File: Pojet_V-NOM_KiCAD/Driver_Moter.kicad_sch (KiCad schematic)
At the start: 3 parts, among them U701 ZXBM5210-SP

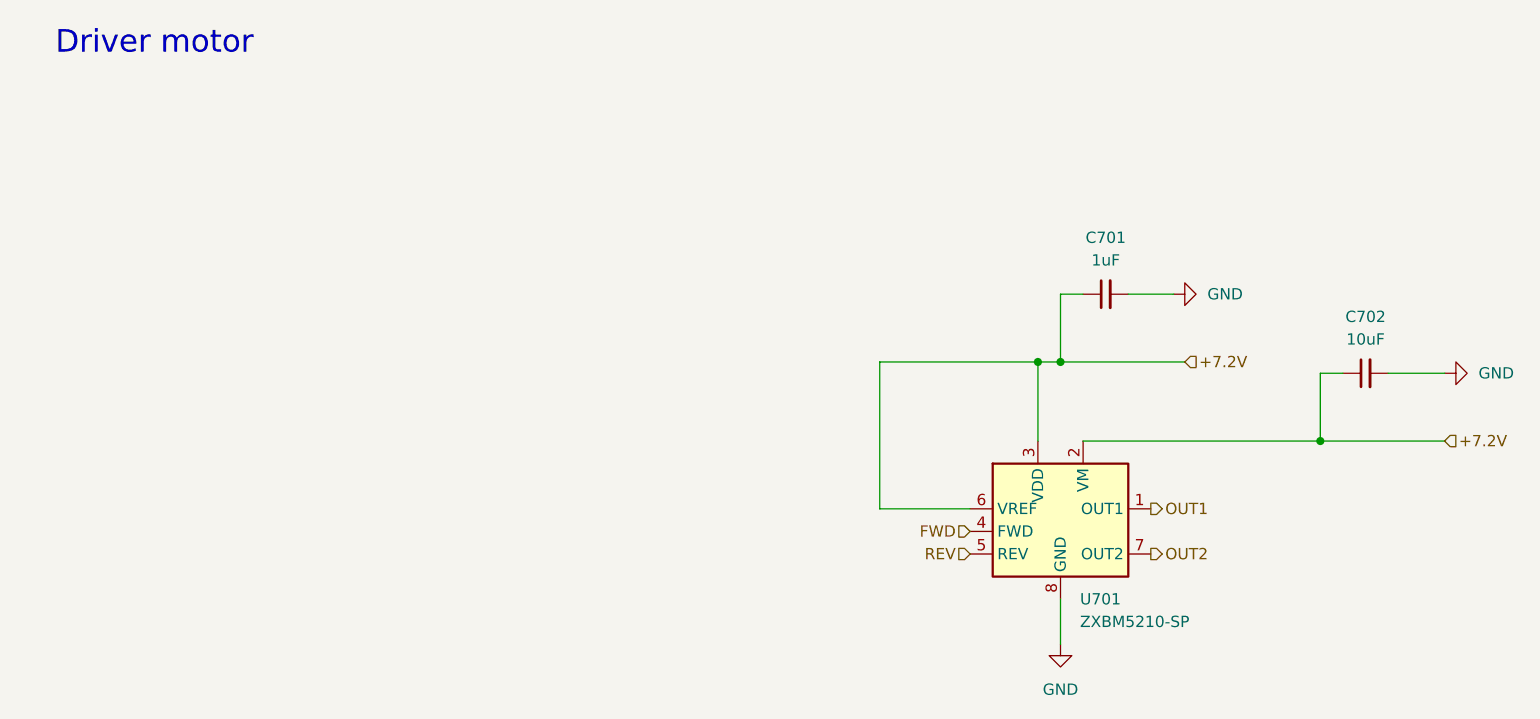
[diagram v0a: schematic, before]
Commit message: Corrections rapides du schéma global
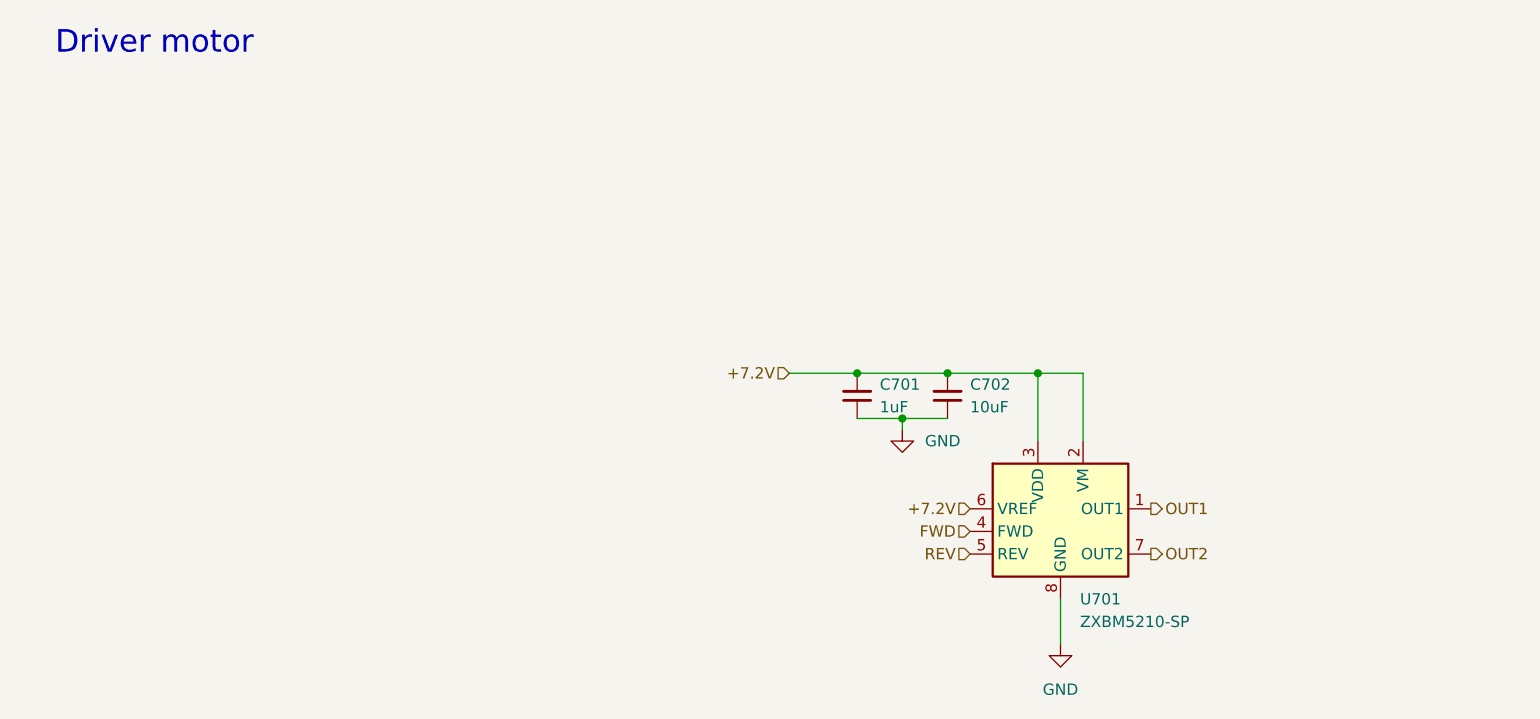
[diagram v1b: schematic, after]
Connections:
- net +7.2V: now also C701.2, C702.2; no longer C701.1, C702.1
- net GND: now also C701.1, C702.1; no longer C701.2, C702.2
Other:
- moved on the sheet: C701, C702
